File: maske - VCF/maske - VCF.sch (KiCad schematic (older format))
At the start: 94 parts

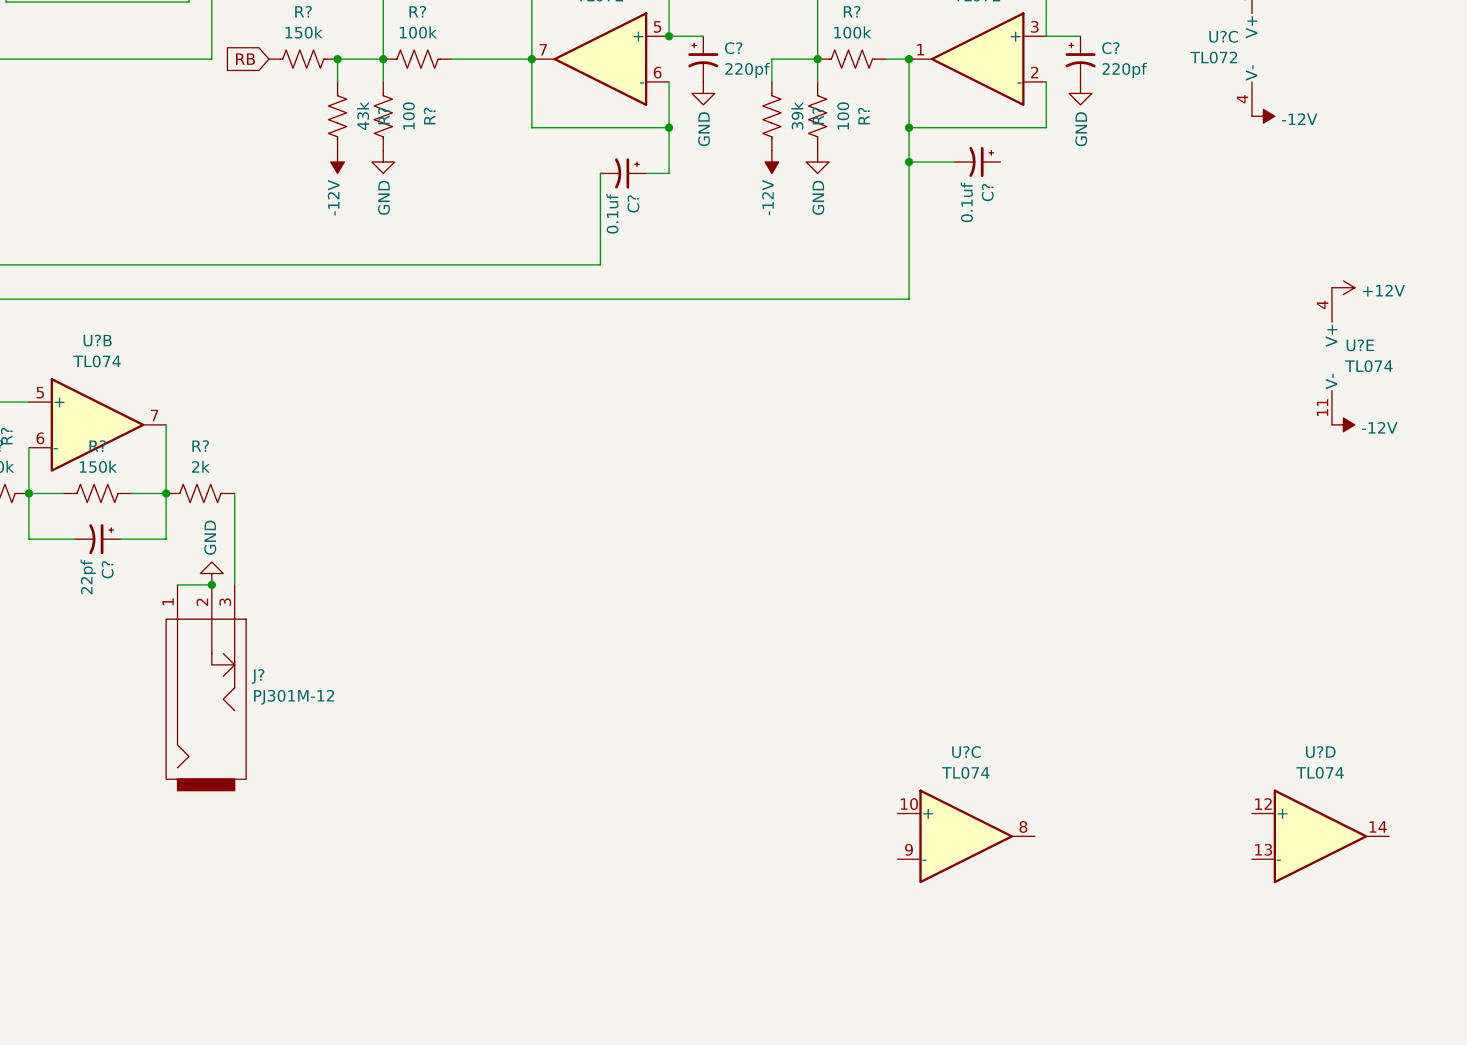
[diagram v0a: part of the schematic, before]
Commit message: m
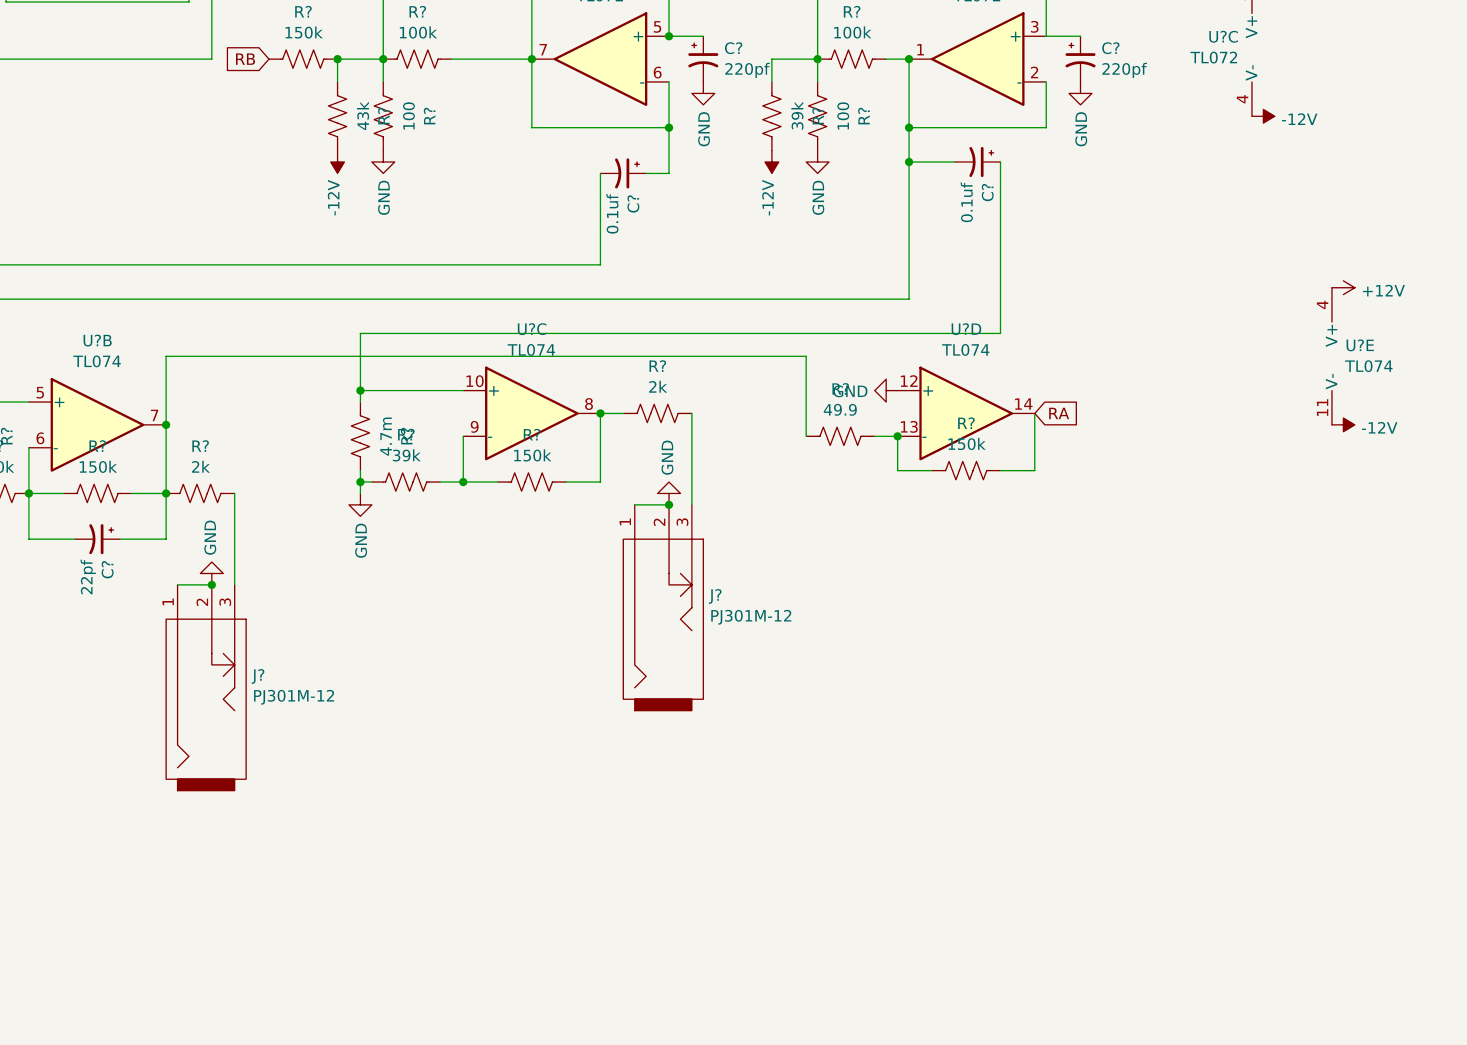
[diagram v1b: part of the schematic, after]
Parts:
- added J?: PJ301M-12, symbol Eurorack:PJ301M-12
- added R?: 2k, symbol Device:R_US
- added R? (x2): 150k, symbol Device:R_US
- added R?: 39k, symbol Device:R_US
- added R?: 4.7m, symbol Device:R_US
- added R?: 49.9, symbol Device:R_US
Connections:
- net GND: now also U?.12 (+), J?.1, J?.2, R?.1, R?.2
- net at C?.1: now also U?.10 (+), R?.2
- net at C?.1, R?.1, R?.2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: now also R?.2
- net at U?.8: now also R?.1, R?.2
- net at U?.9 (-): now also R?.1, R?.2
- net at U?.13 (-): now also R?.1, R?.2
- net RA: now reaches U?.14
- net RA: now also R?.1
- new net: J?.3, R?.1
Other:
- moved on the sheet: U?C, U?D
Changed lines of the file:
@@
 L Amplifier_Operational:TL074 U?
 U 3 1 5D226A27
-P 9400 5400
-F 0 "U?" H 9400 5767 50  0000 C CNN
-F 1 "TL074" H 9400 5676 50  0000 C CNN
-F 2 "" H 9350 5500 50  0001 C CNN
-F 3 "http://www.ti.com/lit/ds/symlink/tl071.pdf" H 9450 5600 50  0001 C CNN
-	3    9400 5400
+P 7500 3550
+F 0 "U?" H 7500 3917 50  0000 C CNN
+F 1 "TL074" H 7500 3826 50  0000 C CNN
+F 2 "" H 7450 3650 50  0001 C CNN
+F 3 "http://www.ti.com/lit/ds/symlink/tl071.pdf" H 7550 3750 50  0001 C CNN
+	3    7500 3550
 	1    0    0    -1
 $EndComp
@@
 L Amplifier_Operational:TL074 U?
 U 4 1 5D226A2D
-P 10950 5400
-F 0 "U?" H 10950 5767 50  0000 C CNN
-F 1 "TL074" H 10950 5676 50  0000 C CNN
-F 2 "" H 10900 5500 50  0001 C CNN
-F 3 "http://www.ti.com/lit/ds/symlink/tl071.pdf" H 11000 5600 50  0001 C CNN
-	4    10950 5400
+P 9400 3550
+F 0 "U?" H 9400 3917 50  0000 C CNN
+F 1 "TL074" H 9400 3826 50  0000 C CNN
+F 2 "" H 9350 3650 50  0001 C CNN
+F 3 "http://www.ti.com/lit/ds/symlink/tl071.pdf" H 9450 3750 50  0001 C CNN
+	4    9400 3550
 	1    0    0    -1
 $EndComp
@@
 	5000 2900 5000 3500
 Connection ~ 5000 3500
+$Comp
+L Device:R_US R?
+U 1 1 5D61A51A
+P 8050 3550
+F 0 "R?" V 7845 3550 50  0000 C CNN
+F 1 "2k" V 7936 3550 50  0000 C CNN
+F 2 "" V 8090 3540 50  0001 C CNN
+F 3 "~" H 8050 3550 50  0001 C CNN
+	1    8050 3550
+	0    1    1    0
+$EndComp
+$Comp
+L Device:R_US R?
+U 1 1 5D61B162
+P 7500 3850
+F 0 "R?" V 7295 3850 50  0000 C CNN
+F 1 "150k" V 7386 3850 50  0000 C CNN
+F 2 "" V 7540 3840 50  0001 C CNN
+F 3 "~" H 7500 3850 50  0001 C CNN
+	1    7500 3850
+	0    1    1    0
+$EndComp
+$Comp
+L Device:R_US R?
+U 1 1 5D61BD45
+P 6950 3850
+F 0 "R?" V 6745 3850 50  0000 C CNN
+F 1 "39k" V 6836 3850 50  0000 C CNN
+F 2 "" V 6990 3840 50  0001 C CNN
+F 3 "~" H 6950 3850 50  0001 C CNN
+	1    6950 3850
+	0    1    1    0
+$EndComp
+$Comp
+L Device:R_US R?
+U 1 1 5D61C559
+P 6750 3650
+F 0 "R?" V 6545 3650 50  0000 C CNN
+F 1 "4.7m" V 6636 3650 50  0000 C CNN
+F 2 "" V 6790 3640 50  0001 C CNN
+F 3 "~" H 6750 3650 50  0001 C CNN
+	1    6750 3650
+	-1   0    0    1
+$EndComp
+$Comp
+L power:GND #PWR?
+U 1 1 5D61D84A
+P 6750 3900
+F 0 "#PWR?" H 6750 3650 50  0001 C CNN
+F 1 "GND" V 6755 3772 50  0000 R CNN
+F 2 "" H 6750 3900 50  0001 C CNN
+F 3 "" H 6750 3900 50  0001 C CNN
+	1    6750 3900
+	1    0    0    -1
+$EndComp
+Wire Wire Line
+	7200 3650 7200 3850
+Wire Wire Line
+	7200 3850 7350 3850
+Wire Wire Line
+	7650 3850 7800 3850
+Wire Wire Line
+	7800 3850 7800 3550
+Wire Wire Line
+	7900 3550 7800 3550
+Connection ~ 7800 3550
+Wire Wire Line
+	7100 3850 7200 3850
+Connection ~ 7200 3850
+Wire Wire Line
+	6750 3900 6750 3850
+Wire Wire Line
+	6750 3850 6800 3850
+Connection ~ 6750 3850
+Wire Wire Line
+	6750 3850 6750 3800
+Wire Wire Line
+	6750 3500 6750 3450
+Wire Wire Line
+	6750 3450 7200 3450
+Wire Wire Line
+	9550 2450 9550 3200
+Wire Wire Line
+	9550 3200 6750 3200
+Wire Wire Line
+	6750 3200 6750 3450
+Connection ~ 6750 3450
+$Comp
+L Eurorack:PJ301M-12 J?
+U 1 1 5D6A4FB0
+P 8100 4400
+F 0 "J?" V 8154 4222 50  0000 R CNN
+F 1 "PJ301M-12" V 8063 4222 50  0000 R CNN
+F 2 "" H 8100 4400 50  0000 C CNN
+F 3 "" H 8100 4400 50  0000 C CNN
+	1    8100 4400
+	0    -1   -1   0
+$EndComp
+Wire Wire Line
+	8200 3950 8200 3550
+Wire Wire Line
+	8100 3950 7950 3950
+$Comp
+L power:GND #PWR?
+U 1 1 5D6A4FB8
+P 8100 3950
+F 0 "#PWR?" H 8100 3700 50  0001 C CNN
+F 1 "GND" V 8105 3822 50  0000 R CNN
+F 2 "" H 8100 3950 50  0001 C CNN
+F 3 "" H 8100 3950 50  0001 C CNN
+	1    8100 3950
+	-1   0    0    1
+$EndComp
+Connection ~ 8100 3950
+$Comp
+L Device:R_US R?
+U 1 1 5D762819
+P 9400 3800
+F 0 "R?" V 9195 3800 50  0000 C CNN
+F 1 "150k" V 9286 3800 50  0000 C CNN
+F 2 "" V 9440 3790 50  0001 C CNN
+F 3 "~" H 9400 3800 50  0001 C CNN
+	1    9400 3800
+	0    1    1    0
+$EndComp
+$Comp
+L Device:R_US R?
+U 1 1 5D763BE6
+P 8850 3650
+F 0 "R?" V 8645 3650 50  0000 C CNN
+F 1 "49.9" V 8736 3650 50  0000 C CNN
+F 2 "" V 8890 3640 50  0001 C CNN
+F 3 "~" H 8850 3650 50  0001 C CNN
+	1    8850 3650
+	0    1    1    0
+$EndComp
+$Comp
+L power:GND #PWR?
+U 1 1 5D764FFF
+P 9100 3450
+F 0 "#PWR?" H 9100 3200 50  0001 C CNN
+F 1 "GND" V 9105 3322 50  0000 R CNN
+F 2 "" H 9100 3450 50  0001 C CNN
+F 3 "" H 9100 3450 50  0001 C CNN
+	1    9100 3450
+	0    1    1    0
+$EndComp
+Wire Wire Line
+	9100 3650 9100 3800
+Wire Wire Line
+	9100 3800 9250 3800
+Wire Wire Line
+	9550 3800 9700 3800
+Wire Wire Line
+	9700 3800 9700 3550
+Wire Wire Line
+	9000 3650 9100 3650
+Connection ~ 9100 3650
+Wire Wire Line
+	5900 3600 5900 3300
+Wire Wire Line
+	5900 3300 8700 3300
+Wire Wire Line
+	8700 3300 8700 3650
+Connection ~ 5900 3600
+Text GLabel 9700 3550 2    50   Input ~ 0
+RA
 $EndSCHEMATC
